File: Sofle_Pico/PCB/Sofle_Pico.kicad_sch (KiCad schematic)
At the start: 78 parts, among them J1 Pimaroni Trackball, J2 4PIN, J3 OLED, J4 OLED, J5 Conn_01x05_Socket, J6 Conn_01x05_Socket, SW1 SW_PUSH_LED, SW10 SW_PUSH_LED, SW11 SW_PUSH_LED, SW12 SW_PUSH_LED, SW13 SW_PUSH_LED, SW14 SW_PUSH_LED, SW15 SW_PUSH_LED, SW16 SW_PUSH_LED, SW17 SW_PUSH_LED, SW18 SW_PUSH_LED, SW19 SW_PUSH_LED, SW2 SW_PUSH_LED, SW20 SW_PUSH_LED, SW21 SW_PUSH_LED, SW22 SW_PUSH_LED, SW23 SW_PUSH_LED, SW24 SW_PUSH_LED, SW25 Rotary_Encoder_Switch, SW26 SW_PUSH_LED, SW27 SW_PUSH_LED, SW28 SW_PUSH_LED, SW29 SW_PUSH_LED, SW3 SW_PUSH_LED, SW30 SW_PUSH_LED, SW4 SW_PUSH_LED, SW5 SW_PUSH_LED, SW6 SW_PUSH_LED, SW7 SW_PUSH_LED, SW8 SW_PUSH_LED, SW9 SW_PUSH_LED, U1 SN74AHCT1G125, U3 Pico

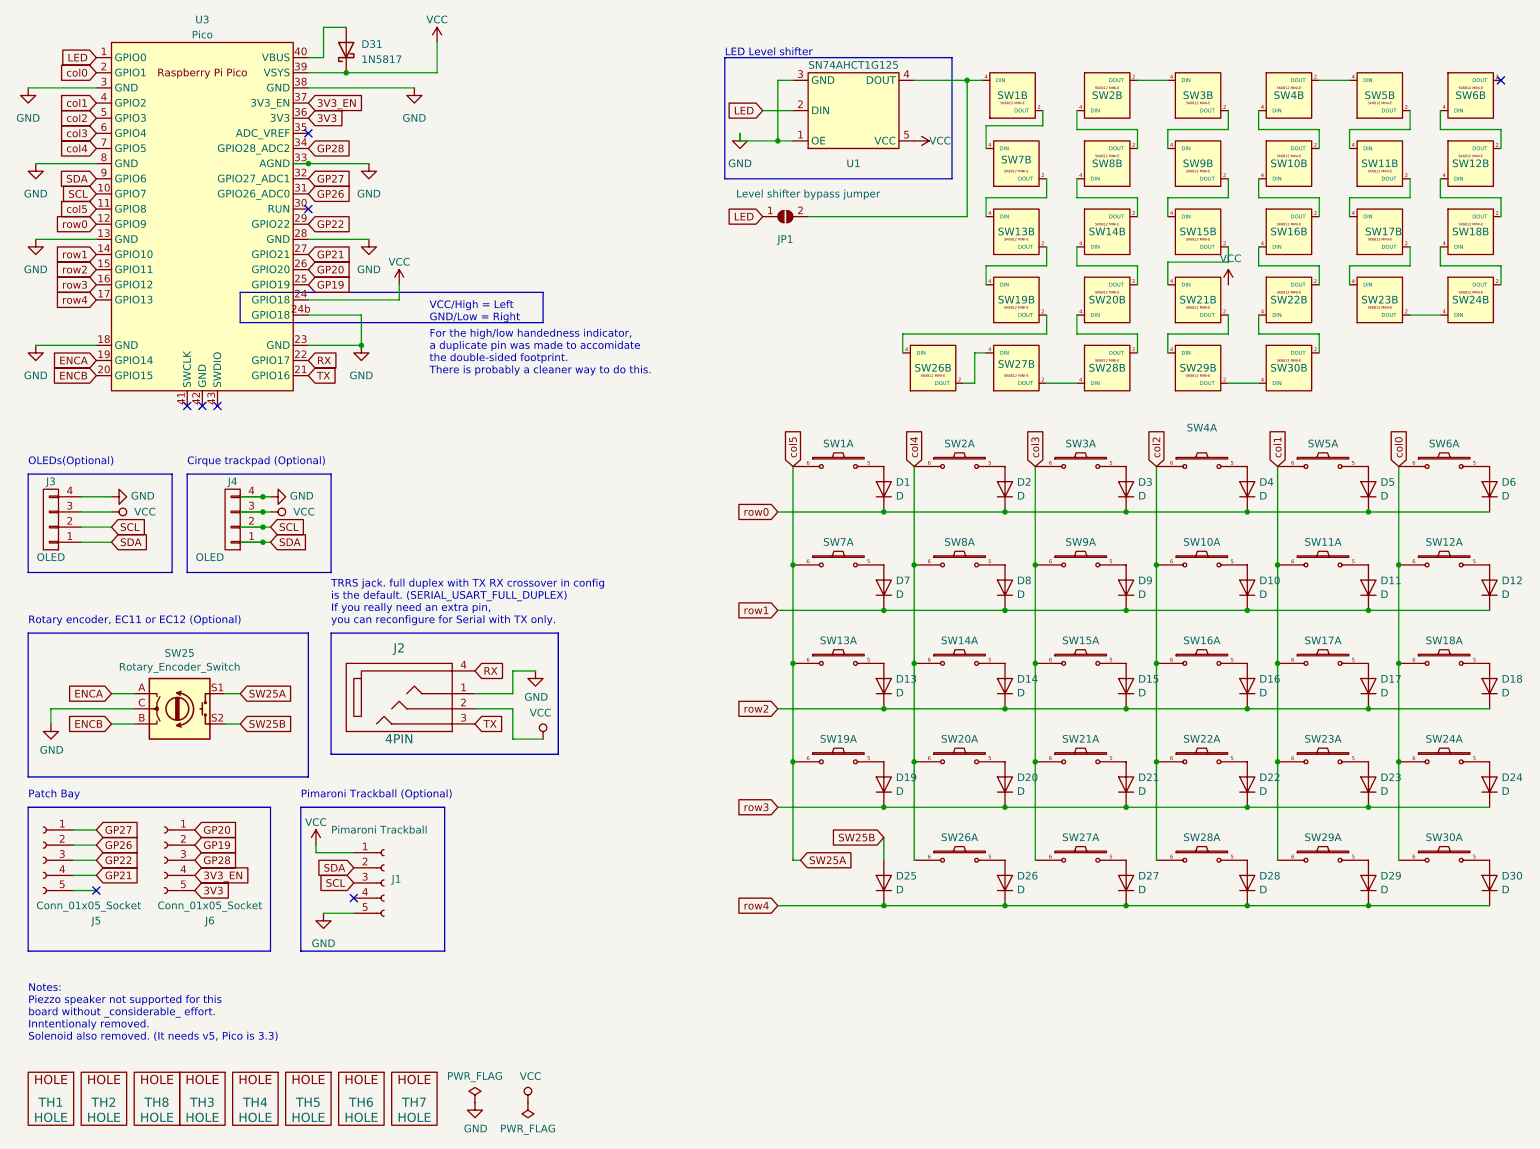
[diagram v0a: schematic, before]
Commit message: Symbol consolidation and cleanup
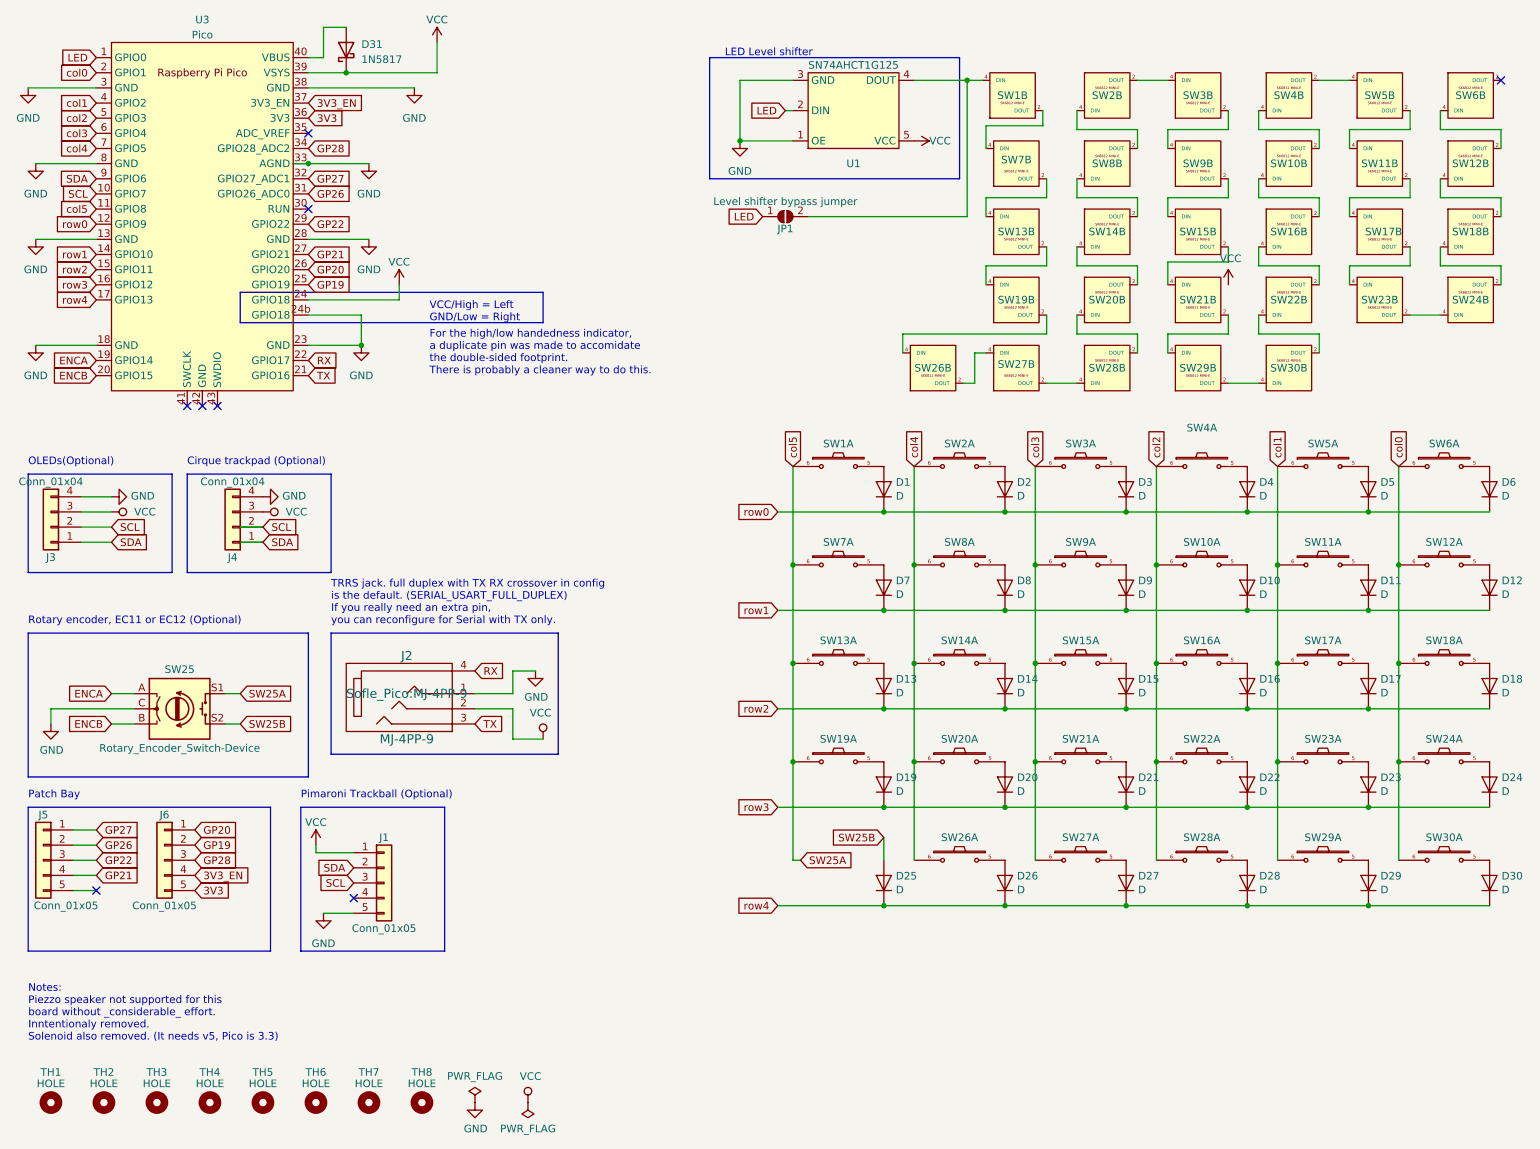
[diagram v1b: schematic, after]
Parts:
- J1: value Pimaroni Trackball -> Conn_01x05; symbol Connector:Conn_01x05_Socket -> Sofle_Pico:Conn_01x05
- J2: value 4PIN -> MJ-4PP-9; symbol SofleKeyboard-rescue:MJ-4PP-9-Lily58-cache-Lily58_Pro-rescue -> Sofle_Pico:MJ-4PP-9
- J3: value OLED -> Conn_01x04; symbol SofleKeyboard-rescue:OLED-Lily58-cache-Lily58_Pro-rescue -> Connector_Generic:Conn_01x04
- J4: value OLED -> Conn_01x04; symbol SofleKeyboard-rescue:OLED-Lily58-cache-Lily58_Pro-rescue -> Sofle_Pico:Conn_01x04
- J5, J6: value Conn_01x05_Socket -> Conn_01x05; symbol Connector:Conn_01x05_Socket -> Sofle_Pico:Conn_01x05
- JP1: value Level shifter bypass jumper -> Level shifter bypass jumper; symbol Jumper:SolderJumper_2_Open -> Sofle_Pico:SolderJumper_2_Open
- SW25: value Rotary_Encoder_Switch -> Rotary_Encoder_Switch-Device; symbol SofleKeyboard-rescue:Rotary_Encoder_Switch-Device -> Sofle_Pico:Rotary_Encoder_Switch-Device
- TH1, TH2, TH3, TH4, TH5, TH6, TH7, TH8: symbol SofleKeyboard-rescue:HOLE-Lily58-cache-Lily58_Pro-rescue -> Sofle_Pico:MountingHole
- U1: footprint Sofle_Pico:SN74AHCT1G125 - Junco -> Sofle_Pico:SN74AHCT1G125; symbol Junco:SN74AHCT1G125 -> Sofle_Pico:SN74AHCT1G125
